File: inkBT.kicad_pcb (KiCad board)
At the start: 2 copper layers, 5.1 x 3.1 mm, 39 parts, among them J1 Conn_01x10, J2 Conn_01x03, J3 Conn_01x02, U1 LM2596S-3.3, U2 ME6211C33M5, U3 ME6211C33M5, U4 LM2596S-5, U5 ESP32-WROOM-32, U6 PCM5102A

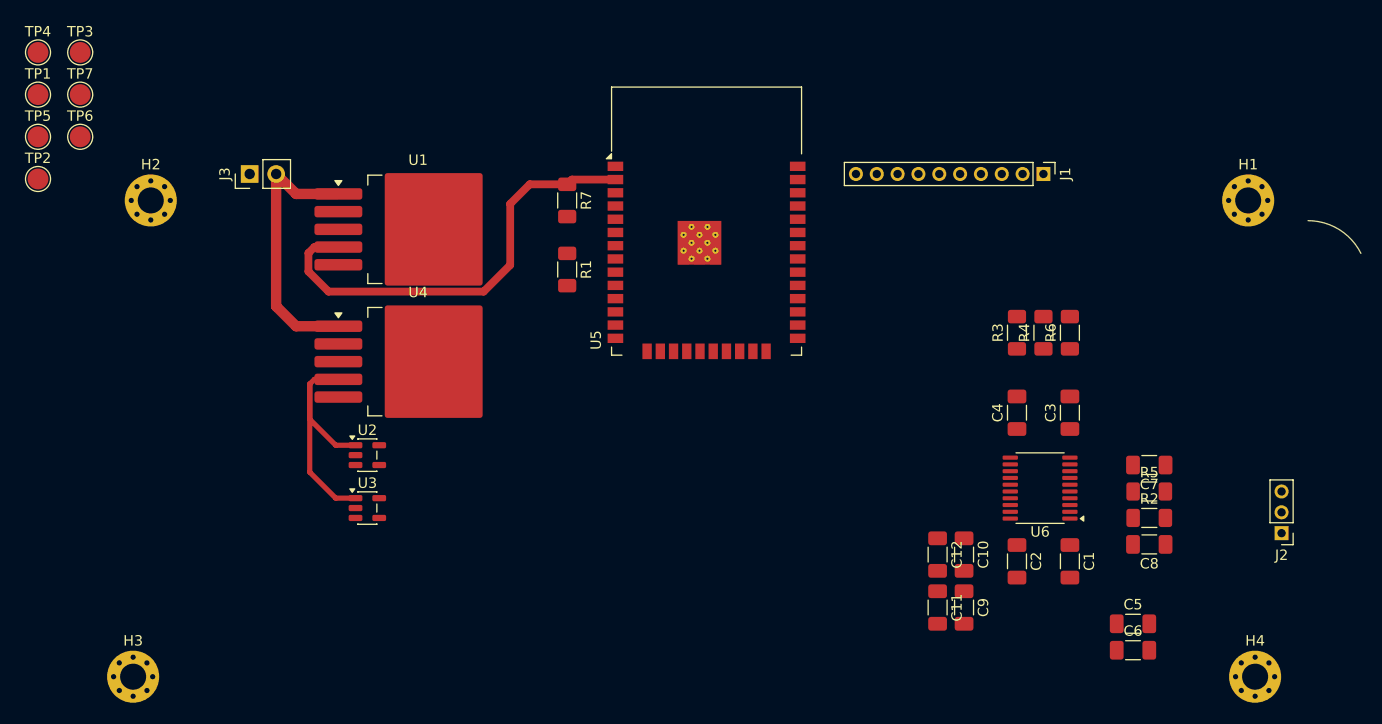
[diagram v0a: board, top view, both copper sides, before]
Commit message: a
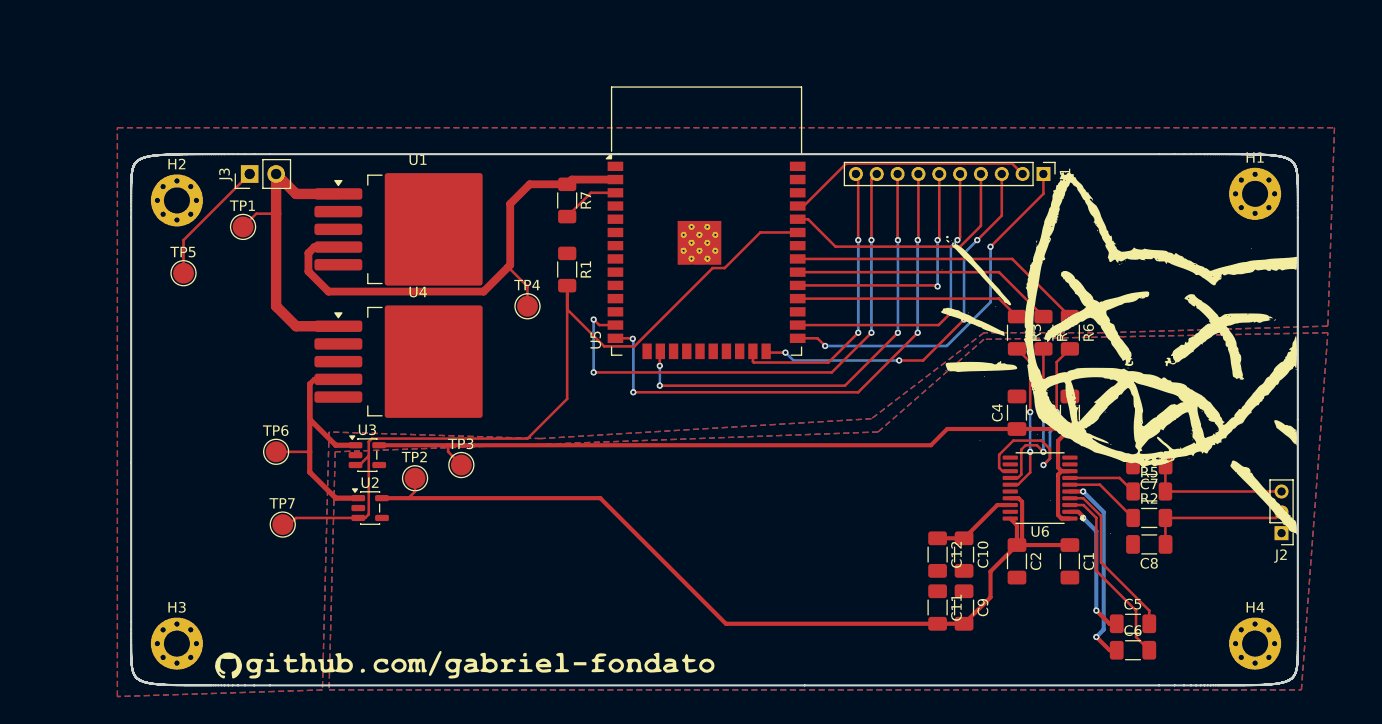
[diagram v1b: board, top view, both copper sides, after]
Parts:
- added ?: LOGO, LOGO, F.Cu at (120.0, 69.8)
- added ?: LOGO, LOGO, F.Cu at (58.4, 100.3)
- added ?: LOGO, LOGO, B.Cu at (45.3, 80.6)
- added ?: LOGO, LOGO, B.Cu at (95.9, 100.3)
- moved TP3 53.9 mm to (58.4, 81.3)
- moved TP4 52.9 mm to (64.8, 66.0)
- moved TP2 46.2 mm to (54.0, 82.5)
- moved TP7 45.6 mm to (41.3, 87.0)
- moved TP6 35.6 mm to (40.6, 80.0)
- moved TP1 23.4 mm to (37.5, 58.4)
- moved TP5 19.1 mm to (31.8, 62.9)
- moved H3 5.27 mm to (31.1, 98.4)
- moved U2 5.09 mm to (49.7, 85.4)
- moved U3 5.08 mm to (49.4, 80.3)
- moved H4 3.17 mm to (134.6, 98.4)
- moved H2 2.51 mm to (31.1, 55.9)
- moved H1 0.92 mm to (134.6, 55.2)
- turned R3 to -90 degrees
- turned R4 to -90 degrees
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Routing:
- net 3.3v Ddac: track 0.00 -> 86.2 mm
- net 3.3v Adac: track 0.00 -> 80.5 mm
- net EN_dac: track 0.00 -> 79.3 mm
- net Net-(J1-Pin_7): track 0.00 -> 51.8 mm, vias 0 -> 4
- net Net-(J1-Pin_9): track 0.00 -> 51.1 mm, vias 0 -> 4
- net Net-(J1-Pin_8): track 0.00 -> 43.5 mm, vias 0 -> 4
- net Net-(J1-Pin_3): track 0.00 -> 36.5 mm, vias 0 -> 4
- net Net-(J1-Pin_1): track 0.00 -> 35.0 mm, vias 0 -> 2
- net Net-(J1-Pin_5): track 0.00 -> 28.9 mm, vias 0 -> 2
- net dac_BCK: track 0.00 -> 28.4 mm
- net Net-(J1-Pin_10): track 0.00 -> 27.7 mm, vias 0 -> 2
- net dac_DIN: track 0.00 -> 25.4 mm
- net Net-(J1-Pin_4): track 0.00 -> 24.5 mm
- net Net-(J1-Pin_6): track 0.00 -> 24.3 mm, vias 0 -> 2
- net Net-(J1-Pin_2): track 0.00 -> 23.7 mm
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- added copper zone on B.Cu, net GND
- added copper zone on F.Cu, net GND
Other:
- board size 5.1 x 3.1 mm -> 112 x 51 mm
